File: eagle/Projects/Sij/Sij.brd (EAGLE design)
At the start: 100 x 80 mm, 9 parts, among them U1 ATMEGA2560AU

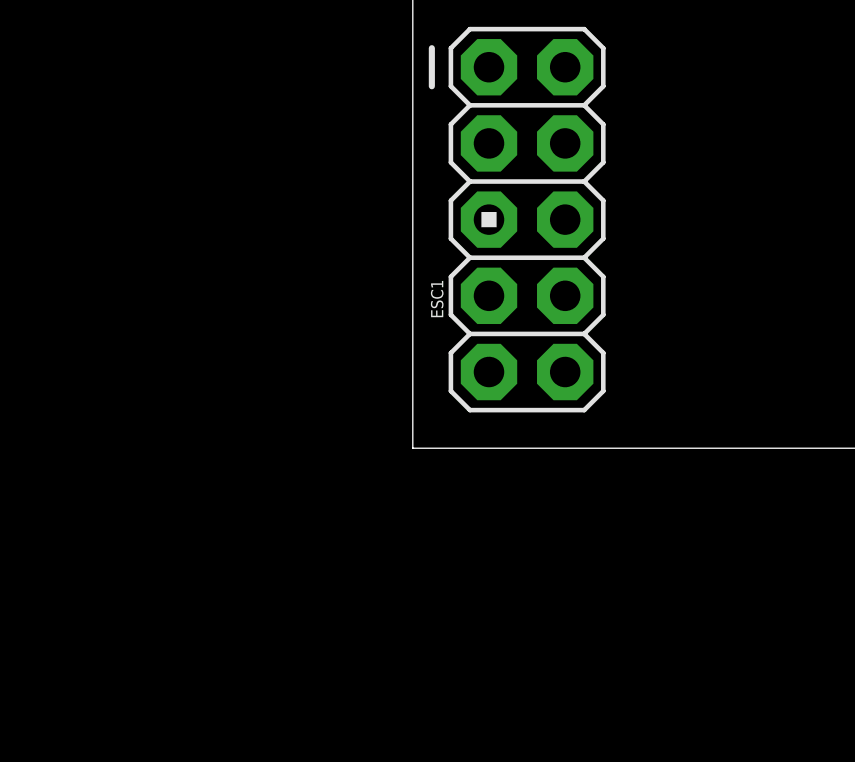
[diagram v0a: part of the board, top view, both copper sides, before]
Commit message: ajouté des pièces pour digikey
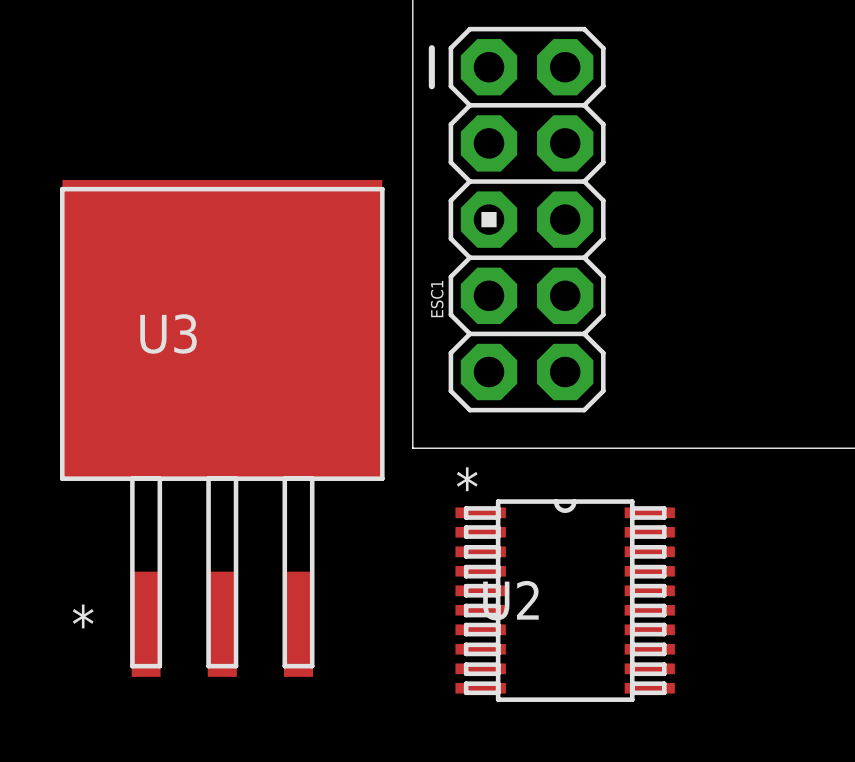
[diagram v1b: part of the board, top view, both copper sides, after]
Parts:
- added U2: BQ76925_PW_20, TI:PW20
- added U3: LM1085_KTT_3, TI:KTT3
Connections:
- new net BAT: U2.2
- new net VSS: U2.10
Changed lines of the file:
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@@
 <attribute name="PROD_ID" value="CAP-07876" x="54.61" y="17.78" size="1.778" layer="27" display="off"/>
+</element>
+<element name="U2" library="TI" package="PW20" value="BQ76925_PW_20" x="5.08" y="-5.08">
+<attribute name="GENERIC_PART_NUMBER" value="BQ76925" x="5.08" y="-5.08" size="1.778" layer="27" display="off"/>
+<attribute name="PACKAGE_DESIGNATOR" value="PW" x="5.08" y="-5.08" size="1.778" layer="27" display="off"/>
+<attribute name="MANUFACTURER" value="Texas Instruments" x="5.08" y="-5.08" size="1.778" layer="27" display="off"/>
+<attribute name="DESCRIPTION" value="Analog Front End for 3 to 6 Series Lithium-Ion Cells" x="5.08" y="-5.08" size="1.778" layer="27" display="off"/>
+<attribute name="VENDOR" value="Texas Instruments" x="5.08" y="-5.08" size="1.778" layer="27" display="off"/>
+<attribute name="INDUSTRY_STD_PKG_TYPE" value="TSSOP" x="5.08" y="-5.08" size="1.778" layer="27" display="off"/>
+<attribute name="FAMILY_NAME" value="LITHIUM ION PROTECTION" x="5.08" y="-5.08" size="1.778" layer="27" display="off"/>
+<attribute name="MANUFACTURER_PART_NUMBER" value="bq76925_pw_20" x="5.08" y="-5.08" size="1.778" layer="27" display="off"/>
+<attribute name="PIN_COUNT" value="20" x="5.08" y="-5.08" size="1.778" layer="27" display="off"/>
+<attribute name="DATASHEETURL" value="http://www.ti.com/lit/gpn/BQ76925" x="5.08" y="-5.08" size="1.778" layer="27" display="off"/>
+</element>
+<element name="U3" library="TI" package="KTT3" value="LM1085_KTT_3" x="-6.35" y="3.81">
+<attribute name="VENDOR" value="Texas Instruments" x="-6.35" y="3.81" size="1.778" layer="27" display="off"/>
+<attribute name="MANUFACTURER_PART_NUMBER" value="lm1085_ktt_3" x="-6.35" y="3.81" size="1.778" layer="27" display="off"/>
 </element>
 </elements>
@@
 <wire x1="45.3" y1="17.78" x2="46.99" y2="22.86" width="0" layer="19" extent="1-1"/>
 </signal>
+<signal name="BAT">
+<contactref element="U2" pad="2"/>
+</signal>
+<signal name="VSS">
+<contactref element="U2" pad="10"/>
+</signal>
 </signals>
